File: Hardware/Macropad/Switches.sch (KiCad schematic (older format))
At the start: 49 parts, among them J2 Conn_01x04_Female, SW1 K40_1U, SW10 K01_1U, SW11 K42_1U, SW12 K32_1U, SW13 K22_1U, SW14 K12_1U, SW15 K02_1U, SW16 K43_1U, SW17 K33_1U, SW18 K23_1U, SW19 K13_1U, SW2 K30_1U, SW20 K03_1U, SW21 Rotary_Encoder_Switch, SW3 K20_1U, SW4 K10_1U, SW5 K00_1U, SW6 K41_1U, SW7 K31_1U, SW8 K21_1U, SW9 K11_1U

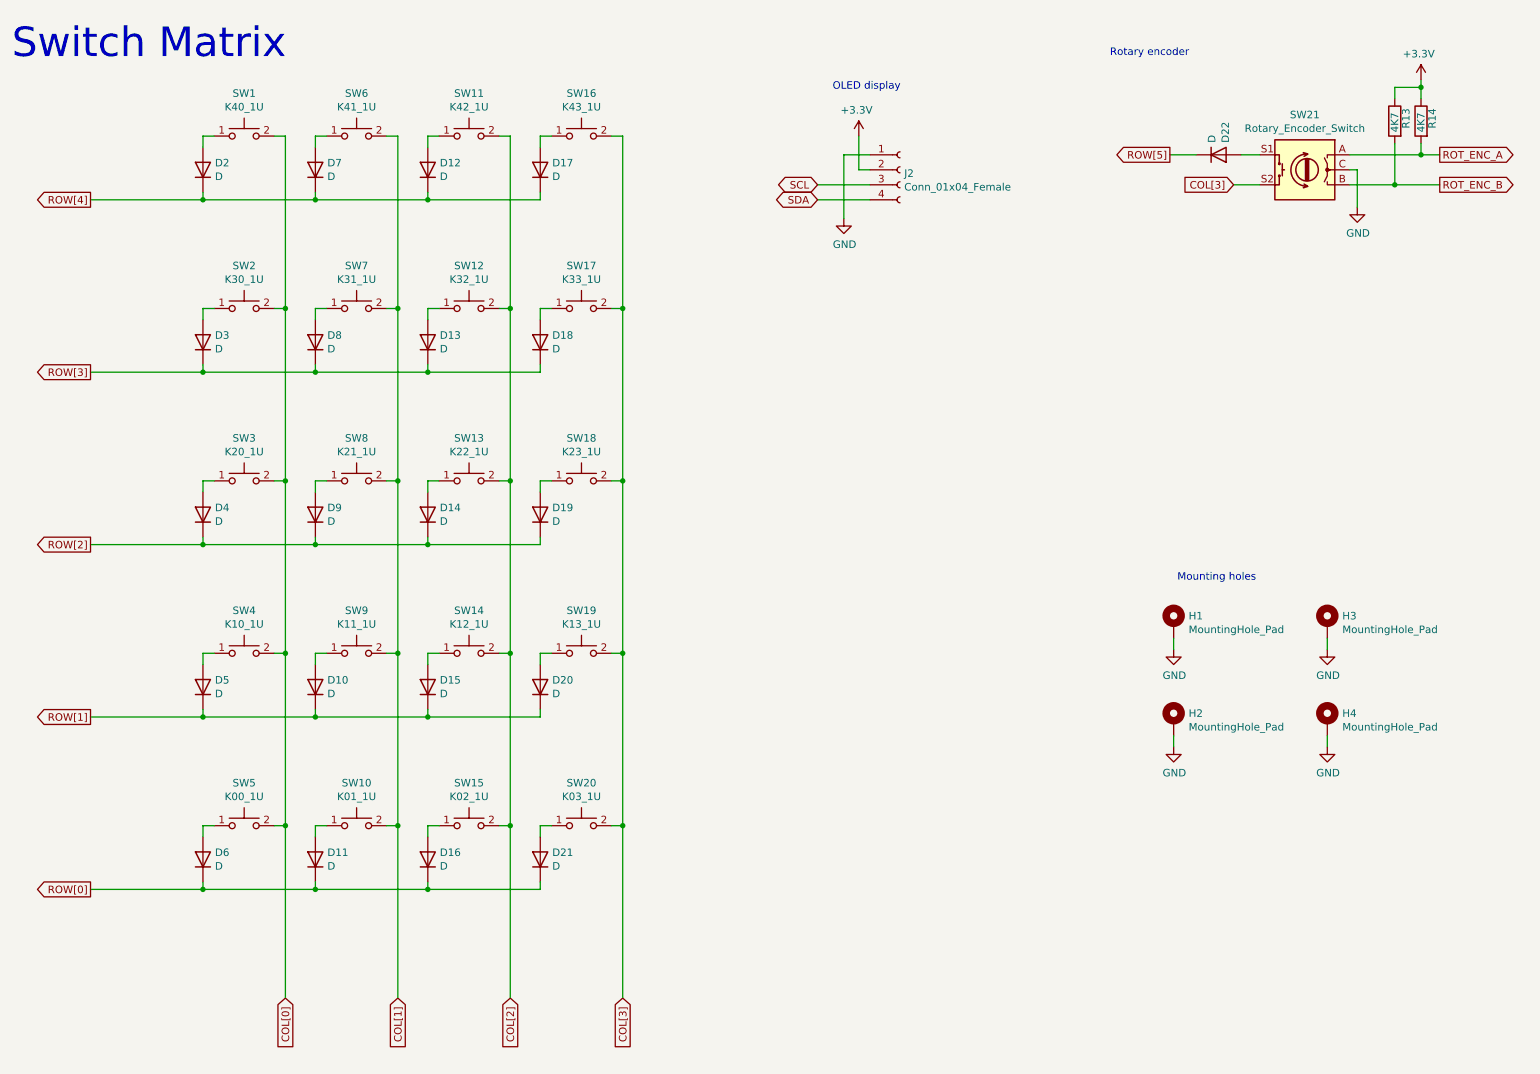
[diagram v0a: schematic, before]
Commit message: Layout done, cleaned up schematic and generated gerbers
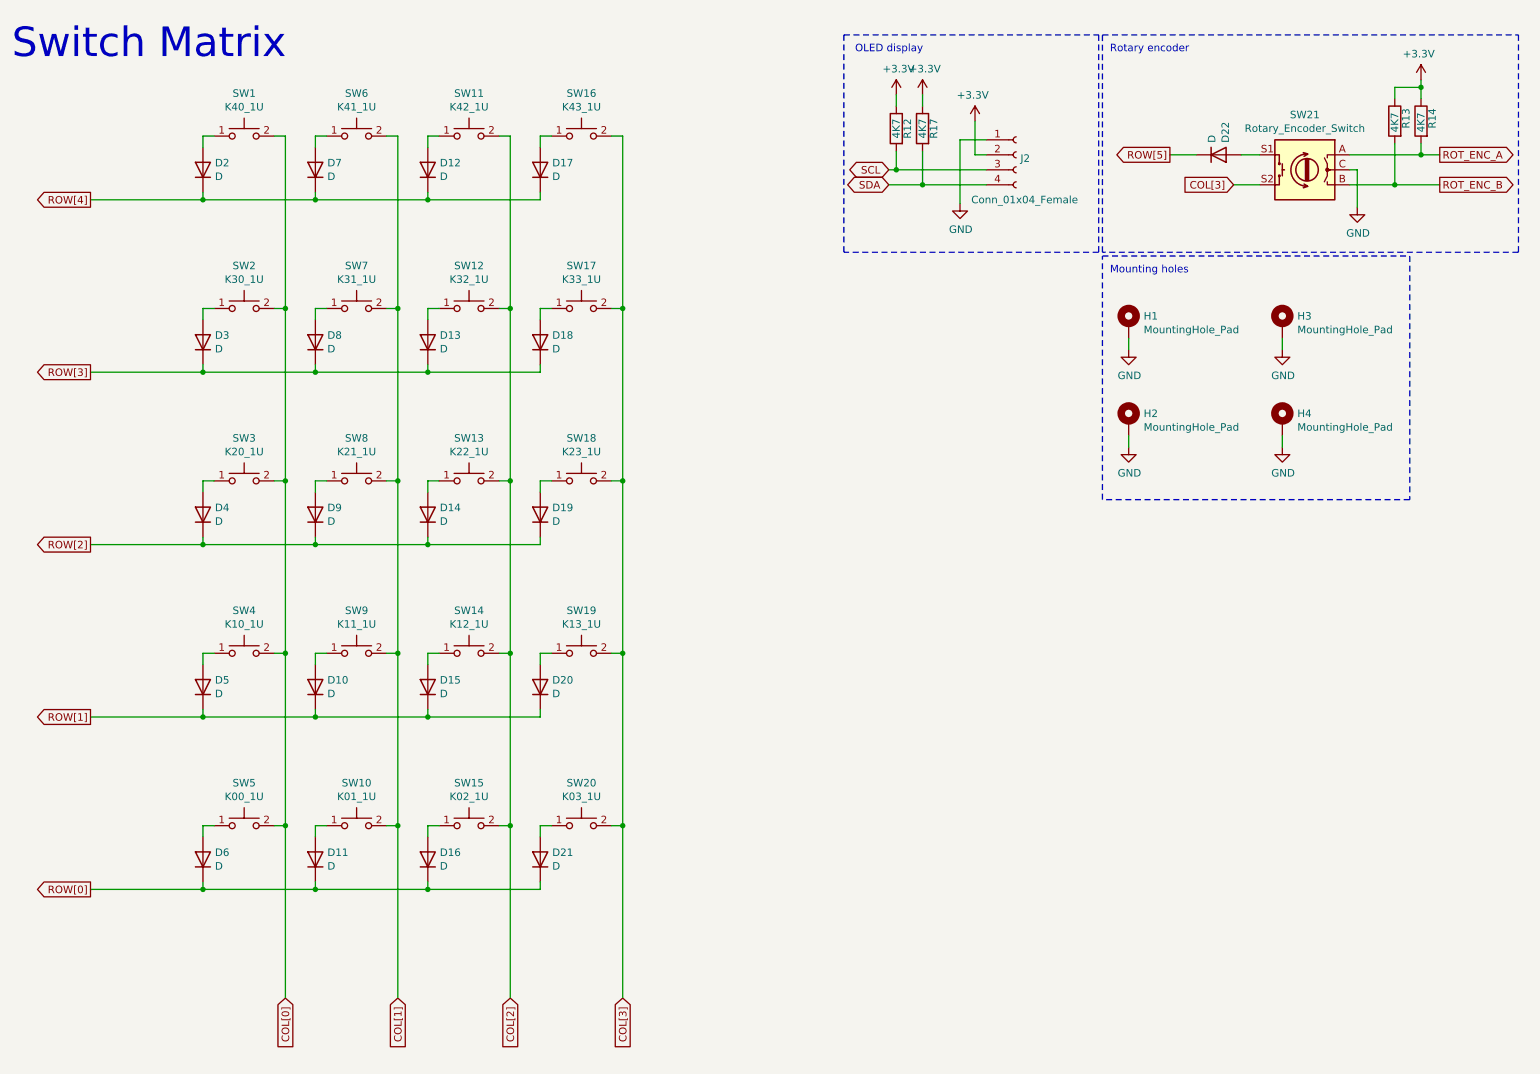
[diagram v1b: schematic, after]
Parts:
- added R12, R17: 4K7, resistor_smd:R_0603_1608Metric, symbol Device:R
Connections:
- net +3V3: now also R12.1, R17.1
- net SCL: now also R12.2
- net SDA: now also R17.2
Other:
- moved on the sheet: H1, H2, H3, H4, J2
